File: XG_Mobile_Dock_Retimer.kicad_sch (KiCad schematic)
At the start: 255 parts, among them J1 5-1775443-8, J13 39301240, J14 469911008, J2 20455-040E-76, J3 20455-040E-76, J7 CEE016400140111, SW1 SW_Push, U1 DS160PT801ACBR, U2 TPS7A8400ARGRR, U7 TPS7A8400ARGRR

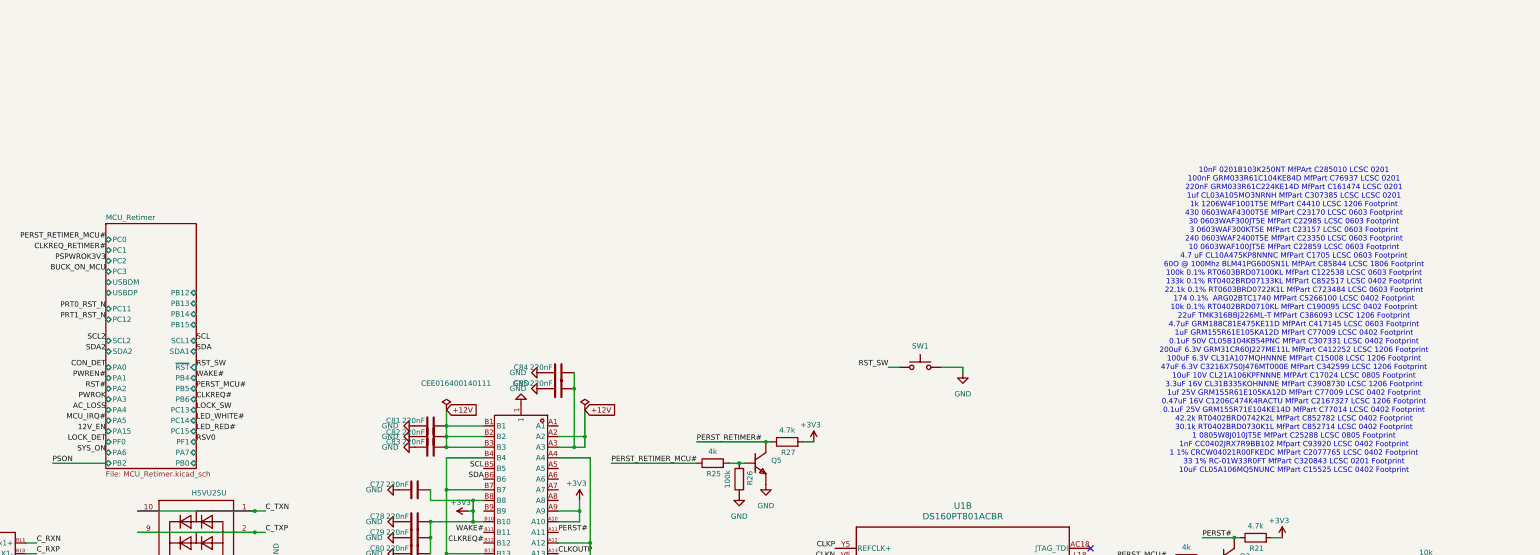
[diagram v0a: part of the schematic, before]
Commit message: eeee
eeee
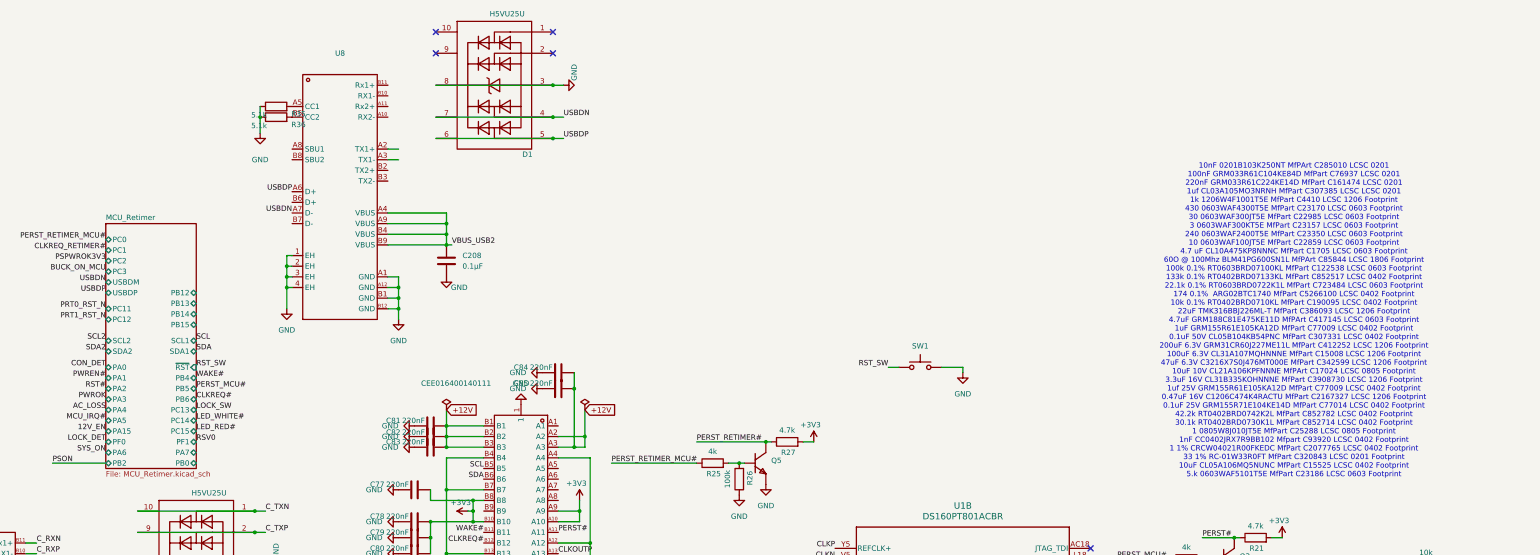
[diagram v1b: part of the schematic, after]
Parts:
- added C208: 0.1μF, Capacitor_SMD:C_0402_1005Metric, symbol Device:C
- added D1: H5VU25U, AZ1045-04F:AZ1045-04F, symbol AZ1045-04F:AZ1045-04F
- added R35, R36: 5.1k, Resistor_SMD:R_0402_1005Metric, symbol Device:R
- added U8: ~, GT-USB-7091A:USB-C-SMD_GT-USB-7091A, symbol GT-USB-7091A:GT-USB-7091A
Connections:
- net GND: now also C208.2, D1.3 (GND), D1.8 (GND), R35.1, R36.1, U8.1 (EH), U8.2 (EH), U8.3 (EH), U8.4 (EH), U8.A1 (GND), U8.A12 (GND), U8.B1 (GND), U8.B12 (GND)
- new net: R36.2, U8.B5 (CC2)
- new net: R35.2, U8.A5 (CC1)
- new net USBDN: D1.4 (I/O_3), D1.7 (NC), U8.A7 (D-)
- new net USBDP: D1.5 (I/O_4), D1.6 (NC), U8.A6 (D+)
- new net VBUS_USB2: C208.1, U8.A4 (VBUS), U8.A9 (VBUS), U8.B4 (VBUS), U8.B9 (VBUS)
- no-connect marks 21 -> 25
